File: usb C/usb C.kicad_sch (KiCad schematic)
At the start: 4 parts

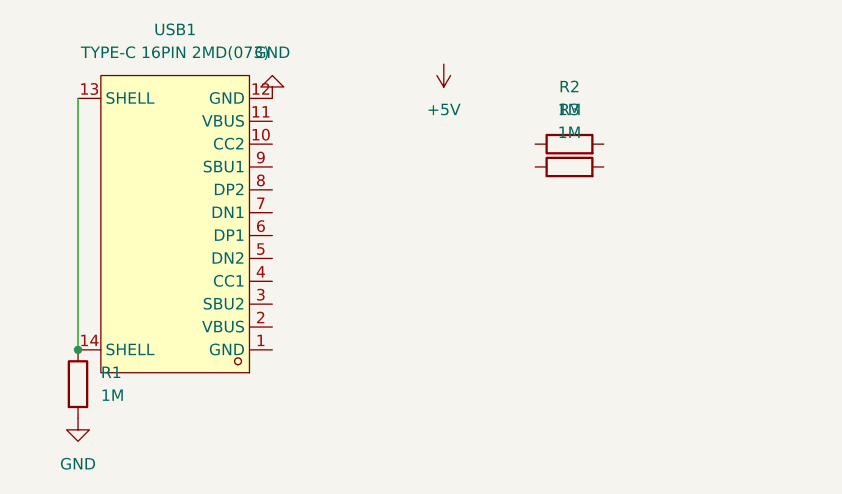
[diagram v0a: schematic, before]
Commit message: pcb
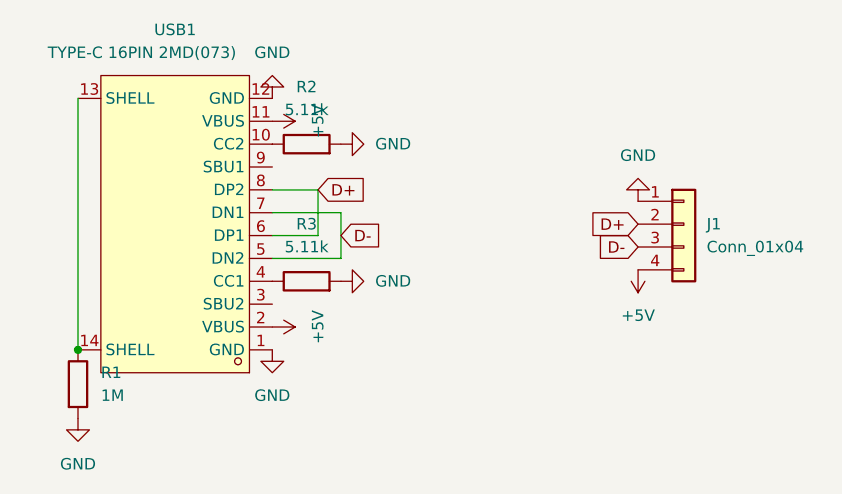
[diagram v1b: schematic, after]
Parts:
- added J1: Conn_01x04, Connector_PinHeader_2.54mm:PinHeader_1x04_P2.54mm_Horizontal, symbol Connector_Generic:Conn_01x04
- R2, R3: value 1M -> 5.11k
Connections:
- net +5V: now also USB1.11 (VBUS), USB1.2 (VBUS), J1.4 (Pin_4)
- net GND: now also R2.2, R3.2, USB1.1 (GND), J1.1 (Pin_1)
- net at USB1.10 (CC2): now also R2.1
- net at USB1.4 (CC1): now also R3.1
- net D-: now reaches USB1.5 (DN2)
- net D-: now also USB1.7 (DN1), J1.3 (Pin_3)
- net D+: now reaches USB1.6 (DP1)
- net D+: now also USB1.8 (DP2), J1.2 (Pin_2)
